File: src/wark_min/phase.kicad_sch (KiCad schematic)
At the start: 32 parts, among them Q301 CJ3439KDW, Q302 IRFH7440TRPBF, Q303 BC846S, Q304 CJ3439KDW, Q305 IRFH7440TRPBF

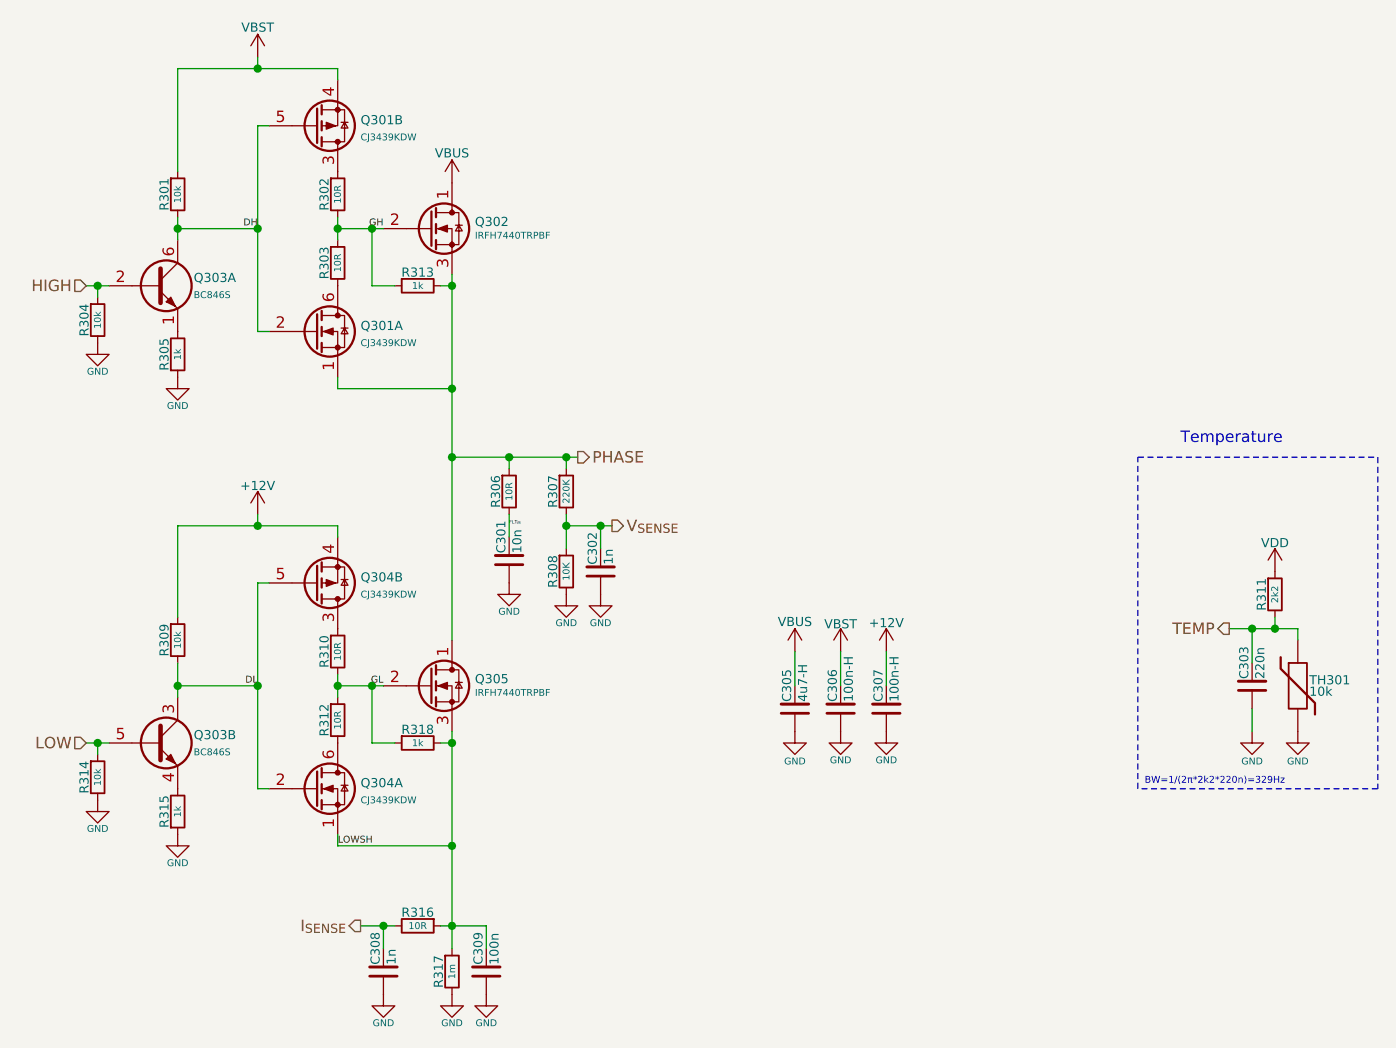
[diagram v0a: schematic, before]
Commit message: Pre-stupid
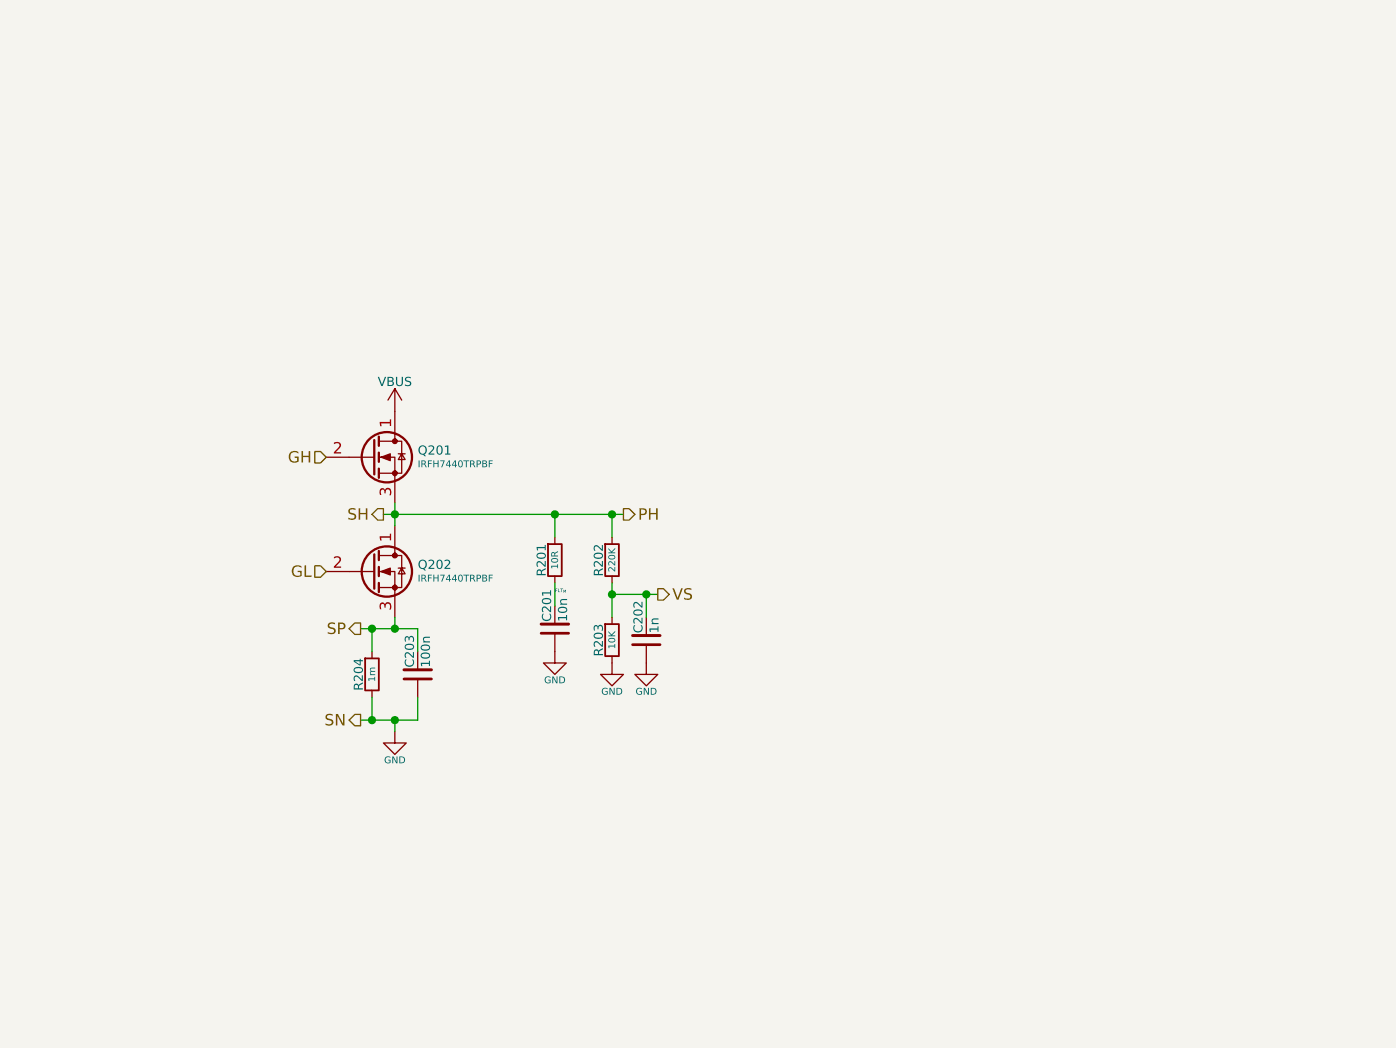
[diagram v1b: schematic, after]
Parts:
- removed C303: 220n, Capacitor_SMD:C_0402_1005Metric, symbol Bluesat:C_CompactV
- removed C305: 4u7-H, Capacitor_SMD:C_1210_3225Metric, symbol Bluesat:C_CompactV
- removed C306, C307: 100n-H, Capacitor_SMD:C_0603_1608Metric, symbol Bluesat:C_CompactV
- removed C308: 1n, Capacitor_SMD:C_0402_1005Metric, symbol Bluesat:C_CompactV
- removed Q301, Q304: CJ3439KDW, Bluesat:SOT-363, symbol Bluesat:DMG1029SV
- removed Q303: BC846S, Bluesat:SOT-363, symbol Transistor_BJT:Q_Dual_NPN_NPN_E1B1C2E2B2C1
- removed R301, R304, R309, R314: 10k, Resistor_SMD:R_0402_1005Metric, symbol Bluesat:R_CompactV
- removed R302, R303, R310, R312, R316: 10R, Resistor_SMD:R_0402_1005Metric, symbol Bluesat:R_CompactV
- removed R305, R313, R315, R318: 1k, Resistor_SMD:R_0402_1005Metric, symbol Bluesat:R_CompactV
- removed R311: 2k2, Resistor_SMD:R_0402_1005Metric, symbol Bluesat:R_CompactV
- removed TH301: 10k, Resistor_SMD:R_0402_1005Metric, symbol Device:Thermistor
- renumbered C301 to C201, C302 to C202, C309 to C203, Q302 to Q201, Q305 to Q202, R306 to R201, R307 to R202, R308 to R203, R317 to R204
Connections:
- net LOWSH renamed SP
- net PHASE renamed PH
- net V_{SENSE} renamed VS
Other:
- note removed: "BW=1/(2π*2k2*220n)=329Hz"
- note removed: "Temperature"
- moved on the sheet: C201, C202, C203, Q201, Q202, R201, R202, R203, R204

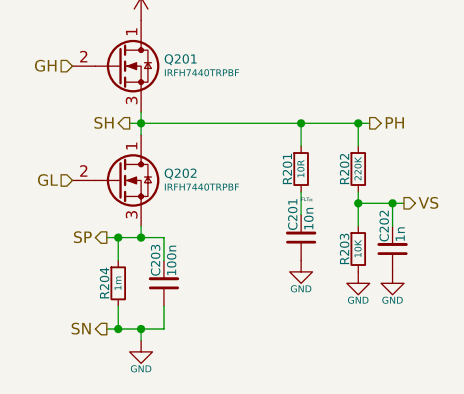
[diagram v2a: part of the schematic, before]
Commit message: Sussy-fus
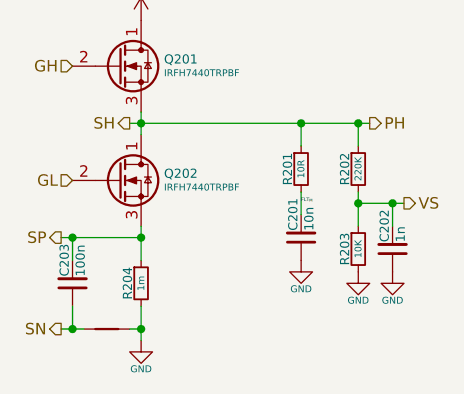
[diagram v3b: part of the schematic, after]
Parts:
- added NT201: NetTie_2, symbol Device:NetTie_2
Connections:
- net GND: now also NT201.2; no longer C203.1
- new net SN: C203.1, NT201.1
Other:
- moved on the sheet: C203, R204
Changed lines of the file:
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@@
+	)
+	(junction
+		(at 49.53 82.55)
+		(diameter 0)
+		(color 0 0 0 0)
 	)
 	(junction
@@
 	)
 	(junction
-		(at 54.61 82.55)
-		(diameter 0)
-		(color 0 0 0 0)
-	)
-	(junction
-		(at 54.61 92.71)
-		(diameter 0)
-		(color 0 0 0 0)
-	)
-	(junction
 		(at 85.09 78.74)
 		(diameter 0)
@@
 	)
 	(junction
+		(at 49.53 92.71)
+		(diameter 0)
+		(color 0 0 0 0)
+	)
+	(junction
 		(at 81.28 69.85)
 		(diameter 0)
@@
 	(wire
 		(pts
-			(xy 54.61 92.71) (xy 57.15 92.71)
-		)
-		(stroke
-			(width 0)
-			(type default)
-		)
-	)
-	(wire
-		(pts
-			(xy 53.34 82.55) (xy 54.61 82.55)
+			(xy 48.26 82.55) (xy 49.53 82.55)
 		)
 		(stroke
@@
 	(wire
 		(pts
-			(xy 54.61 82.55) (xy 54.61 85.09)
+			(xy 49.53 92.71) (xy 50.8 92.71)
+		)
+		(stroke
+			(width 0)
+			(type default)
+		)
+	)
+	(wire
+		(pts
+			(xy 57.15 82.55) (xy 57.15 85.09)
 		)
 		(stroke
@@
 	(wire
 		(pts
-			(xy 59.69 82.55) (xy 59.69 85.09)
-		)
-		(stroke
-			(width 0)
-			(type default)
-		)
-	)
-	(wire
-		(pts
 			(xy 85.09 78.74) (xy 86.36 78.74)
 		)
@@
 	(wire
 		(pts
-			(xy 54.61 82.55) (xy 57.15 82.55)
-		)
-		(stroke
-			(width 0)
-			(type default)
-		)
-	)
-	(wire
-		(pts
 			(xy 55.88 69.85) (xy 57.15 69.85)
 		)
@@
 	(wire
 		(pts
+			(xy 49.53 90.17) (xy 49.53 92.71)
+		)
+		(stroke
+			(width 0)
+			(type default)
+		)
+	)
+	(wire
+		(pts
+			(xy 55.88 92.71) (xy 57.15 92.71)
+		)
+		(stroke
+			(width 0)
+			(type default)
+		)
+	)
+	(wire
+		(pts
 			(xy 81.28 77.47) (xy 81.28 78.74)
 		)
@@
 	(wire
 		(pts
+			(xy 48.26 92.71) (xy 49.53 92.71)
+		)
+		(stroke
+			(width 0)
+			(type default)
+		)
+	)
+	(wire
+		(pts
 			(xy 57.15 92.71) (xy 57.15 93.98)
 		)
@@
 	(wire
 		(pts
-			(xy 53.34 92.71) (xy 54.61 92.71)
+			(xy 49.53 82.55) (xy 57.15 82.55)
+		)
+		(stroke
+			(width 0)
+			(type default)
+		)
+	)
+	(wire
+		(pts
+			(xy 49.53 82.55) (xy 49.53 85.09)
 		)
 		(stroke
@@
 	(wire
 		(pts
-			(xy 57.15 82.55) (xy 59.69 82.55)
-		)
-		(stroke
-			(width 0)
-			(type default)
-		)
-	)
-	(wire
-		(pts
 			(xy 81.28 78.74) (xy 81.28 81.28)
 		)
@@
 	(wire
 		(pts
-			(xy 57.15 92.71) (xy 59.69 92.71)
-		)
-		(stroke
-			(width 0)
-			(type default)
-		)
-	)
-	(wire
-		(pts
 			(xy 74.93 69.85) (xy 81.28 69.85)
 		)
@@
 	(wire
 		(pts
-			(xy 54.61 92.71) (xy 54.61 90.17)
-		)
-		(stroke
-			(width 0)
-			(type default)
-		)
-	)
-	(wire
-		(pts
-			(xy 59.69 90.17) (xy 59.69 92.71)
+			(xy 57.15 92.71) (xy 57.15 90.17)
 		)
 		(stroke
@@
 	(hierarchical_label "SP"
 		(shape output)
-		(at 53.34 82.55 180)
+		(at 48.26 82.55 180)
 		(effects
 			(font
@@
 	(hierarchical_label "SN"
 		(shape output)
-		(at 53.34 92.71 180)
+		(at 48.26 92.71 180)
 		(effects
 			(font
@@
 	(symbol
 		(lib_id "Bluesat:R_CompactV")
-		(at 54.61 87.63 0)
+		(at 57.15 87.63 0)
 		(unit 1)
 		(exclude_from_sim no)
@@
 		(fields_autoplaced yes)
 		(property "Reference" "R204"
-			(at 53.721 87.63 90)
+			(at 56.261 87.63 90)
 			(do_not_autoplace yes)
 			(effects
@@
 		)
 		(property "Value" "1m"
-			(at 54.61 87.63 90)
+			(at 57.15 87.63 90)
 			(do_not_autoplace yes)
 			(effects
@@
 		)
 		(property "Footprint" "Resistor_SMD:R_2512_6332Metric"
-			(at 54.61 87.63 0)
+			(at 57.15 87.63 0)
 			(effects
 				(font
@@
 		)
 		(property "Datasheet" "~"
-			(at 54.61 87.63 0)
+			(at 57.15 87.63 0)
 			(effects
 				(font
@@
 		)
 		(property "Description" "Resistor, compact symbol"
-			(at 54.61 87.63 0)
+			(at 57.15 87.63 0)
 			(effects
 				(font
@@
 	)
 	(symbol
+		(lib_id "Device:NetTie_2")
+		(at 53.34 92.71 0)
+		(unit 1)
+		(exclude_from_sim no)
+		(in_bom no)
+		(on_board yes)
+		(dnp no)
+		(fields_autoplaced yes)
+		(property "Reference" "NT201"
+			(at 53.34 90.17 0)
+			(effects
+				(font
+					(size 1.27 1.27)
+				)
+				(hide yes)
+			)
+		)
+		(property "Value" "NetTie_2"
+			(at 53.34 90.17 0)
+			(effects
+				(font
+					(size 1.27 1.27)
+				)
+				(hide yes)
+			)
+		)
+		(property "Footprint" ""
+			(at 53.34 92.71 0)
+			(effects
+				(font
+					(size 1.27 1.27)
+				)
+				(hide yes)
+			)
+		)
+		(property "Datasheet" "~"
+			(at 53.34 92.71 0)
+			(effects
+				(font
+					(size 1.27 1.27)
+				)
+				(hide yes)
+			)
+		)
+		(property "Description" "Net tie, 2 pins"
+			(at 53.34 92.71 0)
+			(effects
+				(font
+					(size 1.27 1.27)
+				)
+				(hide yes)
+			)
+		)
+		(pin "2"
+		)
+		(pin "1"
+		)
+		(instances
+			(project ""
+				(path "/4290b658-b789-4580-aa76-416e95a5eb26/35de4d11-d03f-4cc6-98bc-b8c2435f85ba"
+					(reference "NT301")
+					(unit 1)
+				)
+				(path "/4290b658-b789-4580-aa76-416e95a5eb26/4d34d922-b5cf-40a9-9b41-7d150c3000ed"
+					(reference "NT401")
+					(unit 1)
+				)
+				(path "/4290b658-b789-4580-aa76-416e95a5eb26/e924291c-21ef-4bdc-a76d-e21a3df7fbbf"
+					(reference "NT201")
+					(unit 1)
+				)
+			)
+		)
+	)
+	(symbol
 		(lib_id "Bluesat:C_CompactV")
 		(at 74.93 82.55 0)
@@
 	(symbol
 		(lib_id "Bluesat:C_CompactV")
-		(at 59.69 87.63 0)
+		(at 49.53 87.63 0)
 		(unit 1)
 		(exclude_from_sim no)
@@
 		(fields_autoplaced yes)
 		(property "Reference" "C203"
-			(at 58.801 86.868 90)
+			(at 48.641 86.868 90)
 			(do_not_autoplace yes)
 			(effects
@@
 		)
 		(property "Value" "100n"
-			(at 60.579 86.868 90)
+			(at 50.419 86.868 90)
 			(do_not_autoplace yes)
 			(effects
@@
 		)
 		(property "Footprint" "Capacitor_SMD:C_0402_1005Metric"
-			(at 59.69 87.63 90)
+			(at 49.53 87.63 90)
 			(effects
 				(font
@@
 		)
 		(property "Datasheet" "~"
-			(at 59.69 87.63 90)
+			(at 49.53 87.63 90)
 			(effects
 				(font
@@
 		)
 		(property "Description" "Unpolarized capacitor, compact symbol"
-			(at 59.69 87.63 0)
-			(effects
-				(font
+			(at 49.53 87.63 0)
+			(effects
+				(font
